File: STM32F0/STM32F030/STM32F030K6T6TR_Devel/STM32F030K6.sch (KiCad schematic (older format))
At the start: 18 parts, among them J3 Conn_02x10_Odd_Even, J6 Conn_02x05 Odd_Even, SW1 SW_Push, SW2 SW_DIP_x02, U1 STM32F030K6Tx, Y1 8MHz

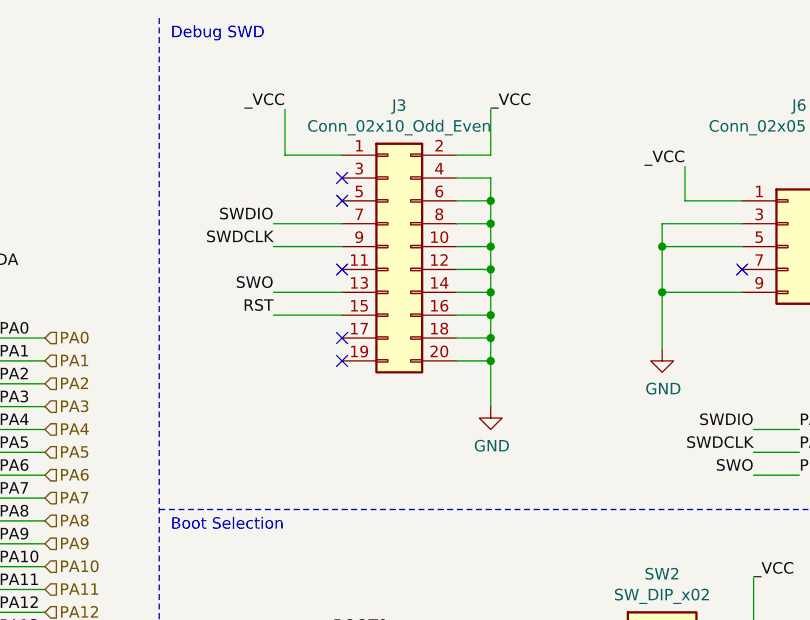
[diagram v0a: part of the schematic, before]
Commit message: F030K6 Board
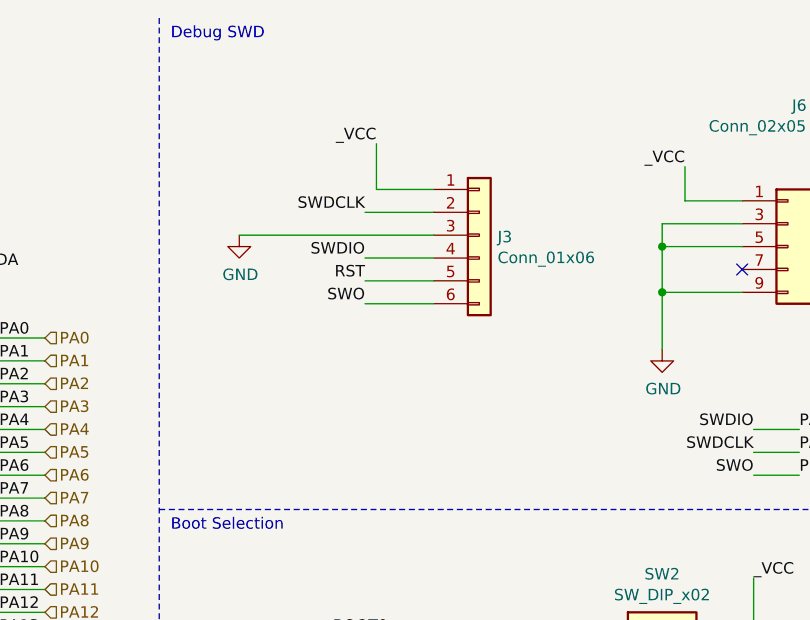
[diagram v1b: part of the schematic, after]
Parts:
- removed J3: Conn_02x10_Odd_Even, Connector_PinHeader_2.54mm:PinHeader_2x10_P2.54mm_Vertical, symbol Connector_Generic:Conn_02x10_Odd_Even
- added J3: Conn_01x06, Connector_PinHeader_2.54mm:PinHeader_1x06_P2.54mm_Vertical, symbol Connector_Generic:Conn_01x06
- J6: footprint Connector_PinHeader_1.27mm:PinHeader_2x05_P1.27mm_Vertical -> Connector_PinHeader_1.27mm:PinHeader_2x05_P1.27mm_Vertical_SMD
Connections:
- net GND: now also J3.3 (Pin_3)
- net NRST: now also J3.5 (Pin_5)
- net PA13: now also J3.4 (Pin_4)
- net PA14: now also J3.2 (Pin_2)
- net PB3: now also J3.6 (Pin_6)
- net VCC: now also J3.1 (Pin_1)
- no-connect marks 9 -> 4
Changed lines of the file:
@@
 	3350 500  3350 5600
-$Comp
-L Connector_Generic:Conn_02x10_Odd_Even J?
-U 1 1 612C8F68
-P 4350 1500
-AR Path="/612C8F68" Ref="J?"  Part="1"
-AR Path="/6115F145/612C8F68" Ref="J3"  Part="1"
-F 0 "J3" H 4400 2117 50  0000 C CNN
-F 1 "Conn_02x10_Odd_Even" H 4400 2026 50  0000 C CNN
-F 2 "Connector_PinHeader_2.54mm:PinHeader_2x10_P2.54mm_Vertical" H 4350 1500 50  0001 C CNN
-F 3 "~" H 4350 1500 50  0001 C CNN
-	1    4350 1500
-	1    0    0    -1
-$EndComp
 $Comp
 L power:GND #PWR?
 U 1 1 612C8F6E
-P 4800 2200
+P 3700 1450
 AR Path="/612C8F6E" Ref="#PWR?"  Part="1"
 AR Path="/6115F145/612C8F6E" Ref="#PWR030"  Part="1"
-F 0 "#PWR030" H 4800 1950 50  0001 C CNN
-F 1 "GND" H 4805 2027 50  0000 C CNN
-F 2 "" H 4800 2200 50  0001 C CNN
-F 3 "" H 4800 2200 50  0001 C CNN
-	1    4800 2200
-	1    0    0    -1
-$EndComp
-Wire Wire Line
-	4650 1200 4800 1200
-Wire Wire Line
-	4800 1200 4800 1300
-Wire Wire Line
-	4650 1100 4800 1100
-Wire Wire Line
-	4800 1100 4800 900
-Wire Wire Line
-	3900 1100 3900 900
-Wire Wire Line
-	4650 1300 4800 1300
-Connection ~ 4800 1300
-Wire Wire Line
-	4800 1300 4800 1400
-Wire Wire Line
-	4650 1400 4800 1400
-Connection ~ 4800 1400
-Wire Wire Line
-	4650 1500 4800 1500
-Wire Wire Line
-	4800 1400 4800 1500
-Connection ~ 4800 1500
-Wire Wire Line
-	4800 1500 4800 1600
-Connection ~ 4800 1600
-Wire Wire Line
-	4800 1600 4800 1700
-Wire Wire Line
-	4650 1600 4800 1600
-Wire Wire Line
-	4650 1700 4800 1700
-Connection ~ 4800 1700
-Wire Wire Line
-	4800 1700 4800 1800
-Wire Wire Line
-	4650 1800 4800 1800
-Connection ~ 4800 1800
-Wire Wire Line
-	4800 1800 4800 1900
-Wire Wire Line
-	4650 1900 4800 1900
-Connection ~ 4800 1900
-Wire Wire Line
-	4800 1900 4800 2000
-Wire Wire Line
-	4650 2000 4800 2000
-Connection ~ 4800 2000
-Wire Wire Line
-	4800 2000 4800 2200
-Wire Wire Line
-	3900 1100 4150 1100
-NoConn ~ 4150 1200
-NoConn ~ 4150 1300
-NoConn ~ 4150 1600
-NoConn ~ 4150 1900
-NoConn ~ 4150 2000
-Text Label 3850 1800 2    50   ~ 0
+F 0 "#PWR030" H 3700 1200 50  0001 C CNN
+F 1 "GND" H 3705 1277 50  0000 C CNN
+F 2 "" H 3700 1450 50  0001 C CNN
+F 3 "" H 3700 1450 50  0001 C CNN
+	1    3700 1450
+	1    0    0    -1
+$EndComp
+Wire Wire Line
+	4300 1250 4300 1050
+Wire Wire Line
+	4300 1250 4550 1250
+Text Label 4250 1650 2    50   ~ 0
 RST
 Wire Wire Line
-	3850 1800 4150 1800
-Text Label 3850 1500 2    50   ~ 0
+	4250 1650 4550 1650
+Text Label 4250 1350 2    50   ~ 0
 SWDCLK
-Text Label 3850 1400 2    50   ~ 0
+Text Label 4250 1550 2    50   ~ 0
 SWDIO
 Wire Wire Line
-	3850 1400 4150 1400
-Wire Wire Line
-	4150 1500 3850 1500
-Text Label 3850 1700 2    50   ~ 0
+	4250 1550 4550 1550
+Wire Wire Line
+	4550 1350 4250 1350
+Text Label 4250 1750 2    50   ~ 0
 SWO
 Wire Wire Line
-	3850 1700 4150 1700
+	4250 1750 4550 1750
 $Comp
 L Connector_Generic:Conn_02x05_Odd_Even J?
@@
 F 0 "J6" H 6150 2117 50  0000 C CNN
 F 1 "Conn_02x05 Odd_Even" H 6150 2026 50  0000 C CNN
-F 2 "Connector_PinHeader_1.27mm:PinHeader_2x05_P1.27mm_Vertical" H 6100 1500 50  0001 C CNN
+F 2 "Connector_PinHeader_1.27mm:PinHeader_2x05_P1.27mm_Vertical_SMD" H 6100 1500 50  0001 C CNN
 F 3 "~" H 6100 1500 50  0001 C CNN
 	1    6100 1500
@@
 Text Label 5650 1150 2    50   ~ 0
 _VCC
-Text Label 4800 900  0    50   ~ 0
-_VCC
-Text Label 3900 900  2    50   ~ 0
+Text Label 4300 1050 2    50   ~ 0
 _VCC
 Text HLabel 7800 700  0    50   Input ~ 0
@@
 $EndComp
 Connection ~ 7300 3550
+$Comp
+L Connector_Generic:Conn_01x06 J3
+U 1 1 61316A9B
+P 4750 1450
+F 0 "J3" H 4830 1442 50  0000 L CNN
+F 1 "Conn_01x06" H 4830 1351 50  0000 L CNN
+F 2 "Connector_PinHeader_2.54mm:PinHeader_1x06_P2.54mm_Vertical" H 4750 1450 50  0001 C CNN
+F 3 "~" H 4750 1450 50  0001 C CNN
+	1    4750 1450
+	1    0    0    -1
+$EndComp
+Wire Wire Line
+	3700 1450 4550 1450
 $EndSCHEMATC
